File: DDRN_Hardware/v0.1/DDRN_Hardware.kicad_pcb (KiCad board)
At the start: 2 copper layers, 32 x 54 mm, 49 parts, among them J2 Conn_Coaxial, J3 Conn_01x02_Pin, J4 Conn_01x04_Pin, J5 Conn_01x06_Pin, J8 Conn_02x05_Top_Bottom, Q1 BSS119, Q2 BSS119, SW1 SW_Push, U1 LoRa-E5, U2 MAX1932, U3 BMP390L, U4 W25Q32JVSS, U5 LSM303AGR, U6 AP2112K-3.3

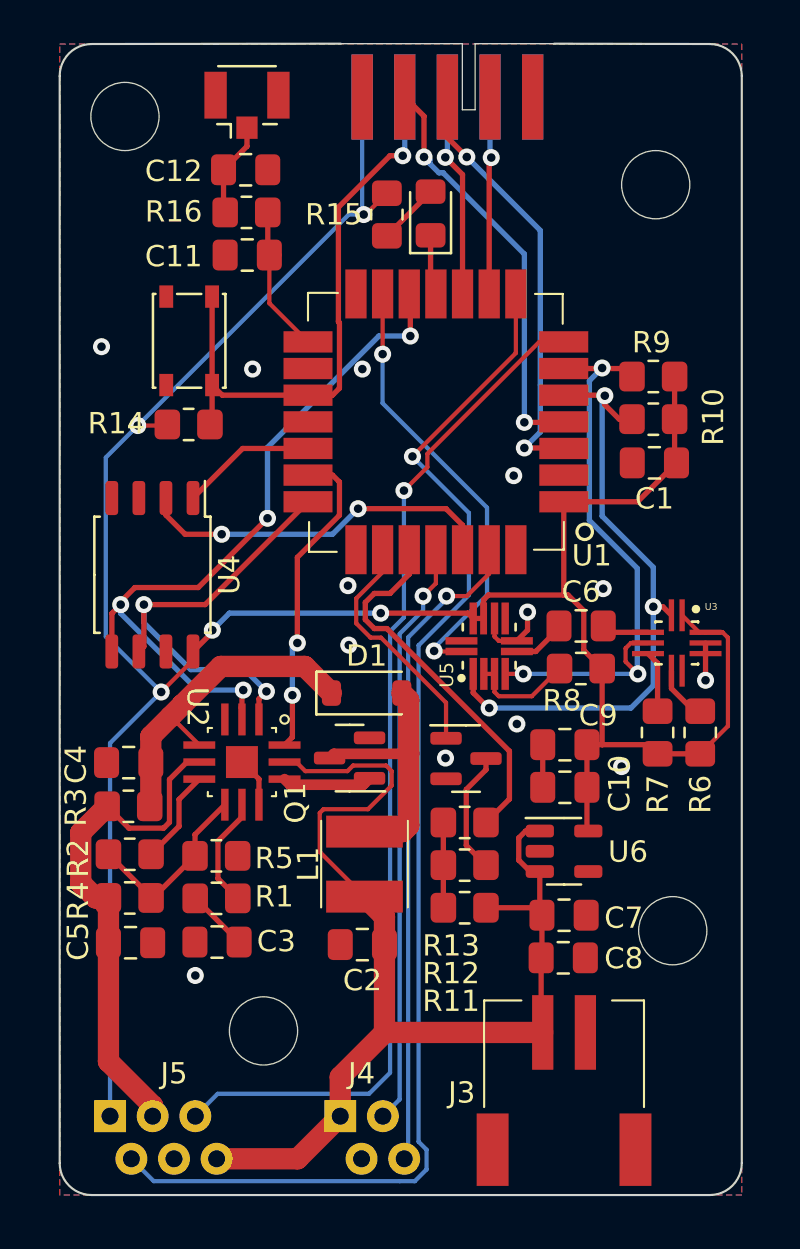
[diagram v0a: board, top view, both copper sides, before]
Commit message: moving files
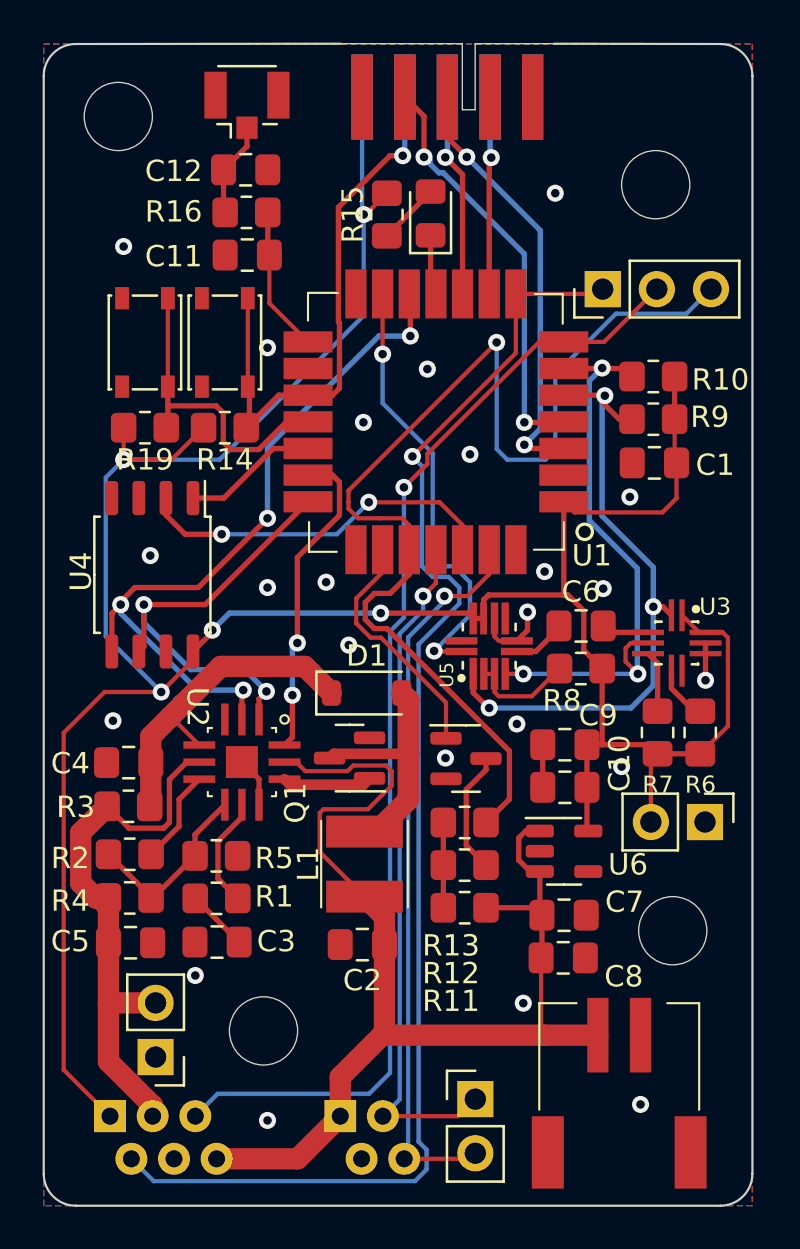
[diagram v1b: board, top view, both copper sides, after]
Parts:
- added J1: Conn_01x03_Pin, Connector_PinHeader_2.54mm:PinHeader_1x03_P2.54mm_Vertical, F.Cu at (79.6, 103.0)
- added J6: Conn_01x02_Pin, Connector_PinHeader_2.54mm:PinHeader_1x02_P2.54mm_Vertical, F.Cu at (58.6, 139.0)
- added J7: Conn_01x02_Pin, Connector_PinHeader_2.54mm:PinHeader_1x02_P2.54mm_Vertical, F.Cu at (73.6, 140.9)
- added J9: Conn_01x02_Pin, Connector_PinHeader_2.54mm:PinHeader_1x02_P2.54mm_Vertical, F.Cu at (84.4, 128.0)
- added R19: 1k, Resistor_SMD:R_0805_2012Metric_Pad1.20x1.40mm_HandSolder, F.Cu at (58.1, 109.5)
- added SW2: SW_Push, Button_Switch_SMD:SW_SPST_PTS810, F.Cu at (58.1, 105.5)
- moved J3 2.59 mm to (80.3, 137.9)
- moved R14 1.71 mm to (61.9, 109.5)
- moved SW1 1.68 mm to (61.9, 105.5)
- moved H2 0.31 mm to (56.9, 94.8)
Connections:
- U1 pad 18: unconnected-(U1-PA3-Pad18) -> /Boot_Mode
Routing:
- net /Battery_Monitor: track 17.7 -> 53.3 mm, vias 0 -> 1
- net /Boot_Mode: track 0.00 -> 14.9 mm
- net /3v3: track 120.6 -> 135.4 mm
- net /SiPM_Signal: track 48.5 -> 53.7 mm
- net /Stim_Enable: track 27.6 -> 32.3 mm
- net /SiPM_Temp: track 59.8 -> 64.1 mm
- net /Anneal_Enable: track 30.8 -> 34.3 mm
- net /V_BAT: track 54.2 -> 56.8 mm
- net /SiPM_Bias: track 24.0 -> 26.2 mm
- net /RST: track 27.7 -> 26.5 mm
- net Net-(D1-A): track 12.3 -> 11.6 mm
- net GND: vias 13 -> 23
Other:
- board size 32 x 54 mm -> 33.3 x 54.5 mm
- board text added: "30v!!!"
- board text added: "3v3"
- board text added: "Anneal_Enable"
- board text added: "Battery_Monitor"
- board text added: "Bias"
- board text added: "GND"
- board text added: "SiPM_SIGNAL"
- board text added: "SiPM_TEMP"
- board text added: "Stim_Enable"
